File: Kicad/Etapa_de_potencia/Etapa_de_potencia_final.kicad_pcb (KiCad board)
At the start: 2 copper layers, 73 parts, among them J1 Conn_01x01_Male, J10 Conn_01x01_Male, J11 Conn_01x01_Male, J12 Conn_01x01_Male, J13 Conn_01x01_Male, J2 Conn_01x01_Male, J3 Conn_01x01_Male, J4 Conn_01x02_Male, J5 Conn_01x01_Male, J6 Conn_01x01_Male, J7 Conn_01x01_Male, J8 Screw_Terminal_01x02, Q1 BC547, Q2 BC557, Q3 BC557, Q4 IRF510, Q5 IRF510, U1 TL084, U2 TLV3501AID, U3 OPA365AID, U4 LM393, U5 IRS20957S, U6 TI-ETD49-2350

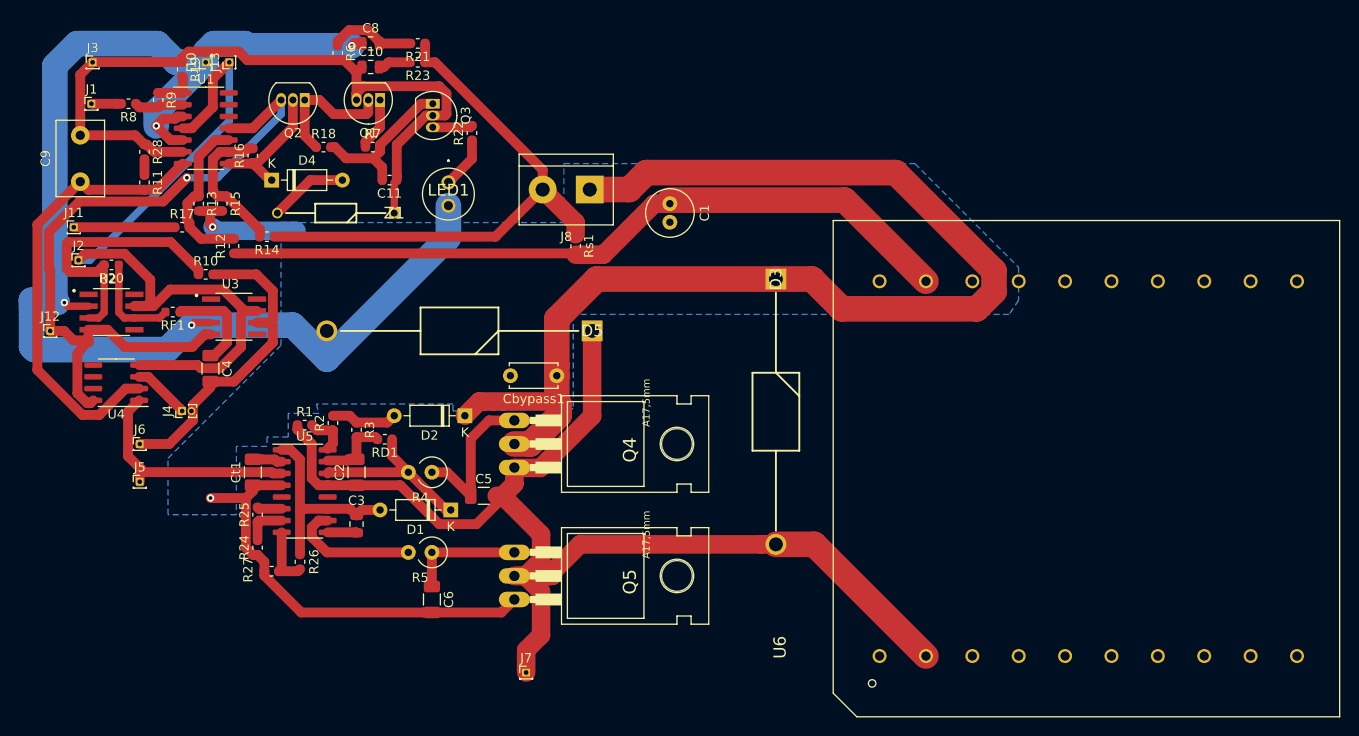
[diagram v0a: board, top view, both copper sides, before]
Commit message: KICAD
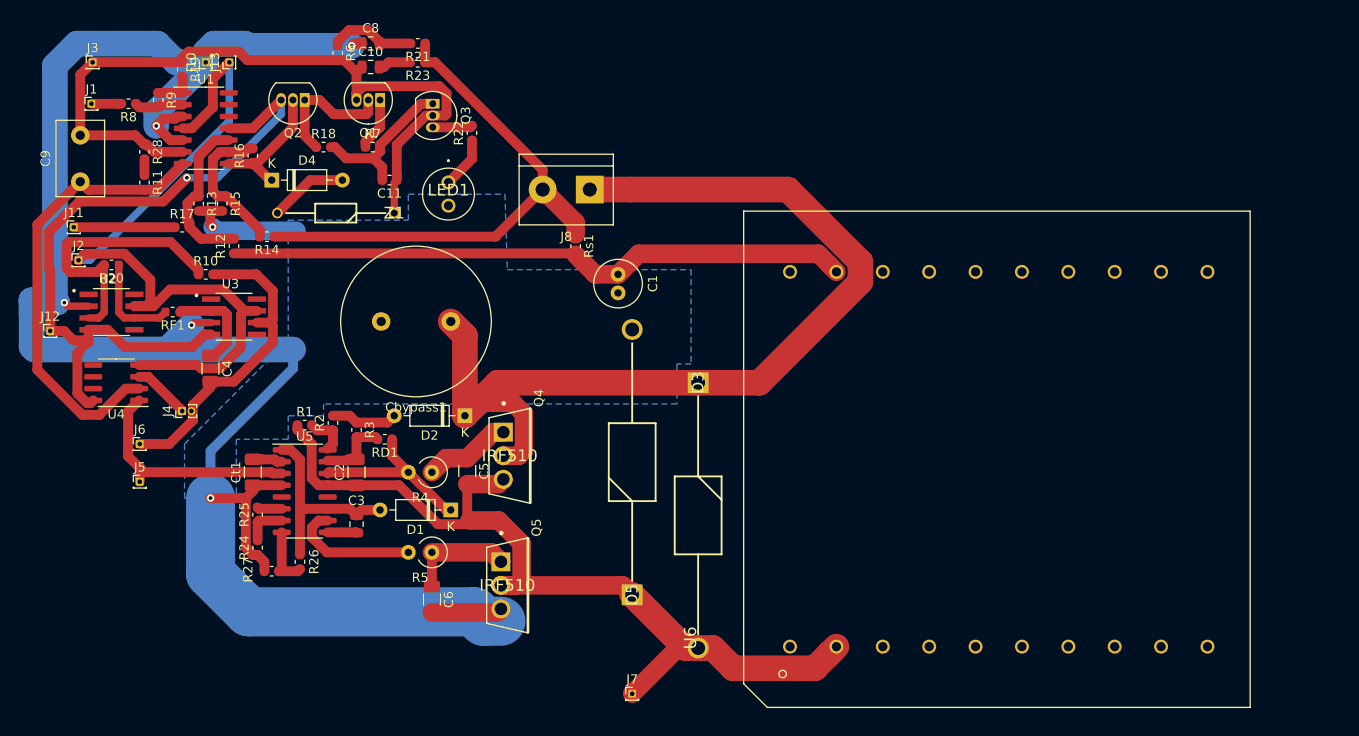
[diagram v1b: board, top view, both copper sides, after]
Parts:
- Cbypass1: value 22u -> 1000u; footprint Capacitor_THT:C_Disc_D5.0mm_W2.5mm_P5.00mm -> Capacitor_THT:C_Radial_D16.0mm_H25.0mm_P7.50mm
- Q4, Q5: footprint IRF510:TO220 -> eec:Vishay-IRF510-0
- moved D5 28.8 mm to (123.7, 97.5), turned to 90 degrees
- moved D3 14.0 mm to (130.8, 74.7)
- moved Cbypass1 12.8 mm to (104.1, 68.1)
- moved J7 11.7 mm to (123.7, 108.2)
- moved U6 9.71 mm to (140.7, 103.1)
- moved C1 9.45 mm to (122.2, 63.0)
- moved Q5 7.18 mm to (110.2, 96.5), turned to 0 degrees
- moved Q4 6.97 mm to (110.5, 82.5), turned to 0 degrees
- moved C5 3.20 mm to (105.9, 84.2), turned to 270 degrees
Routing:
- net Net-(C2-Pad1): track 129.8 -> 96.5 mm
- net VD: track 129.1 -> 105.8 mm
- net GND: track 208.0 -> 222.7 mm
- net Net-(C1-Pad1): track 80.5 -> 67.6 mm
- net Net-(C5-Pad1): track 16.9 -> 9.49 mm
- net Net-(C6-Pad1): track 12.6 -> 11.5 mm
